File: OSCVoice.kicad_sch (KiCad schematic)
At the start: 26 parts, among them U10 TL074, U9 SSI2131

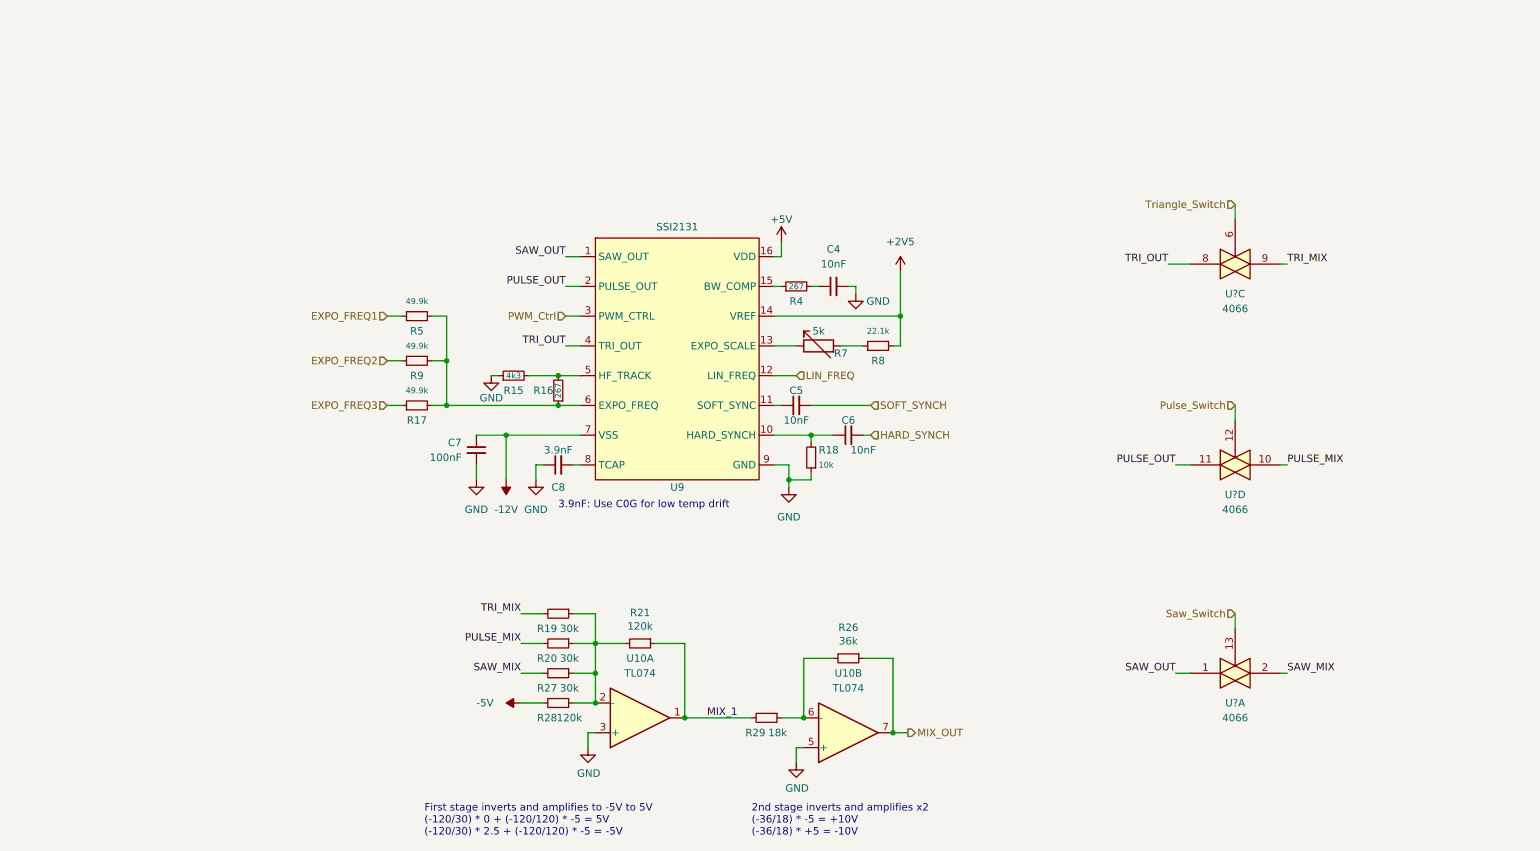
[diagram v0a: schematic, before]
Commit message: Voice schematic work; need to do linear FM
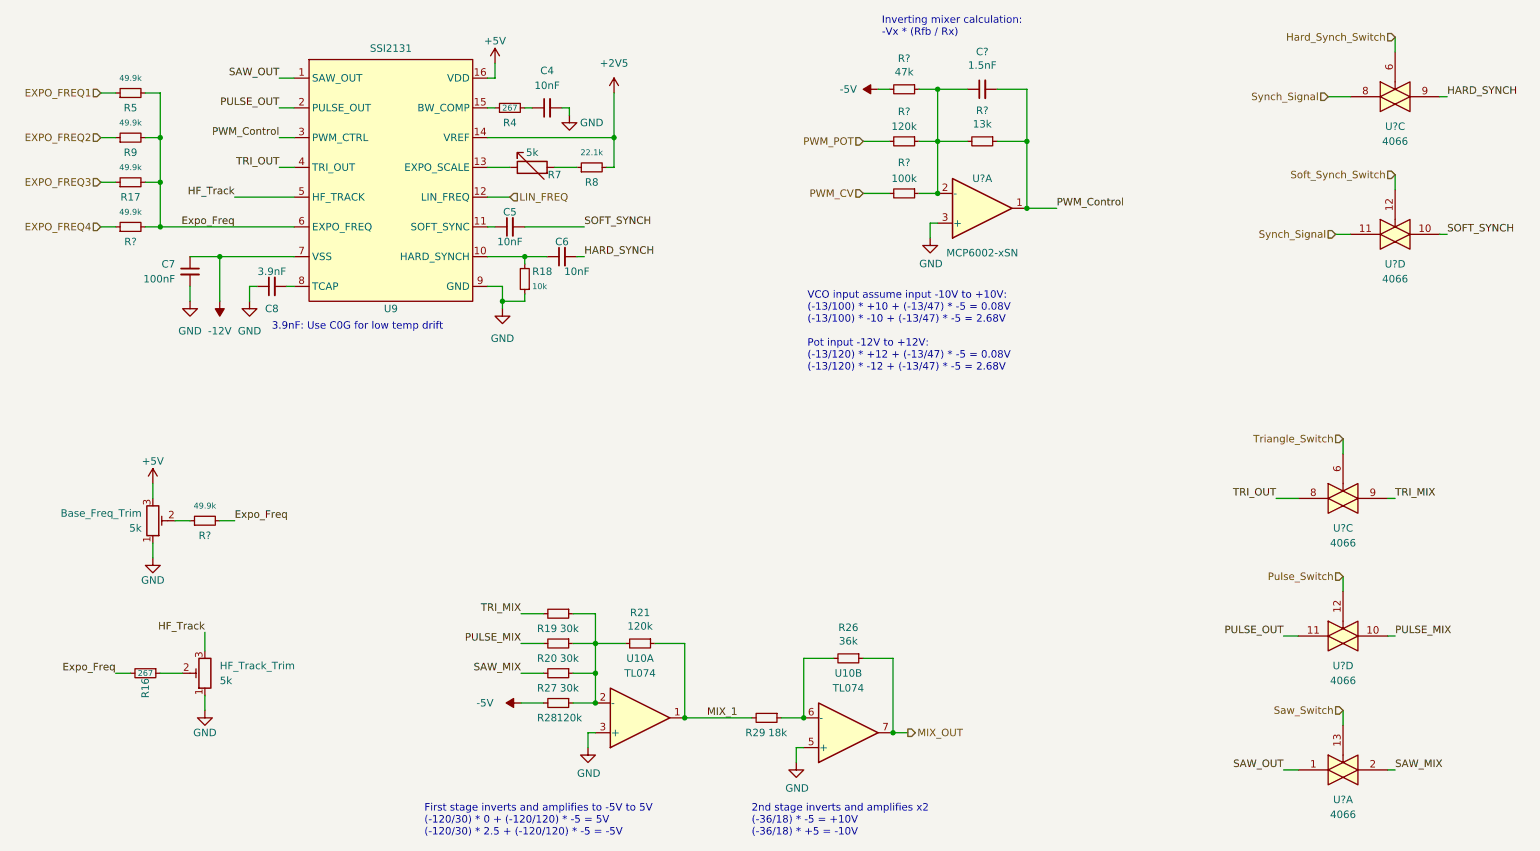
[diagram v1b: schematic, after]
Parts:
- removed R15: 4k3, Resistor_SMD:R_0805_2012Metric, symbol Device:R_Small
- added Base_Freq_Trim, HF_Track_Trim: 5k, Potentiometer_THT:Potentiometer_Bourns_3266W_Vertical, symbol Device:R_Potentiometer_Trim
- added C?: 1.5nF, Capacitor_SMD:C_0805_2012Metric, symbol Device:C_Small
- added R?: 47k, Resistor_SMD:R_0805_2012Metric, symbol Device:R_Small
- added R?: 120k, Resistor_SMD:R_0805_2012Metric, symbol Device:R_Small
- added R? (x2): 49.9k, Resistor_SMD:R_0805_2012Metric, symbol Device:R_Small
- added R?: 13k, Resistor_SMD:R_0805_2012Metric, symbol Device:R_Small
- added R?: 100k, Resistor_SMD:R_0805_2012Metric, symbol Device:R_Small
- added U? (x2): 4066, Package_SO:TSSOP-14_4.4x5mm_P0.65mm, symbol 4xxx:4066
- added U?: MCP6002-xSN, Package_SO:MSOP-8_3x3mm_P0.65mm, symbol Amplifier_Operational:MCP6002-xSN
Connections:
- net +5V: now also Base_Freq_Trim.3
- net -5V: now also R?.2
- net GND: now also Base_Freq_Trim.1, HF_Track_Trim.1, U?.3 (+)
- net HARD_SYNCH: now also U?.9
- net SOFT_SYNCH: now also U?.10
- net Expo_Freq: now reaches R17.2, R5.2, R9.2, U9.6 (EXPO_FREQ)
- net Expo_Freq: now also R16.2, R?.2, R?.2; no longer R16.1
- net HF_Track: now reaches U9.5 (HF_TRACK)
- net HF_Track: now also HF_Track_Trim.3; no longer R16.2
- net PWM_Ctrl renamed PWM_Control
- net PWM_Control: now also C?.2, R?.1, U?.1
- new net: C?.1, R?.1, R?.1, R?.1, R?.2, U?.2 (-)
- new net: HF_Track_Trim.2, R16.1
- new net: Base_Freq_Trim.2, R?.1
- new net EXPO_FREQ4: R?.1
- new net Hard_Synch_Switch: U?.6
- new net PWM_CV: R?.2
- new net PWM_POT: R?.2
- new net Soft_Synch_Switch: U?.12
- new net Synch_Signal: U?.11, U?.8
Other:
- note added: "Inverting mixer calculation: -Vx * (Rfb / Rx)"
- note added: "VCO input assume input -10V to +10V: (-13/100) * +10 + (-13/47) * -5 = 0.08V (-13/100) * -10 + (-13/47) * -5 = 2.68V Pot input -12V to +12V: (-13/120) * +12 + (-13/47) * -5 = 0.08V (-13/120) * -12 + (-13/47) * -5 = 2.68V"
- moved on the sheet: C4, C5, C6, C7, C8, R16, R17, R18, R4, R5, R7, R8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
